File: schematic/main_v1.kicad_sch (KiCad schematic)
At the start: 12 parts

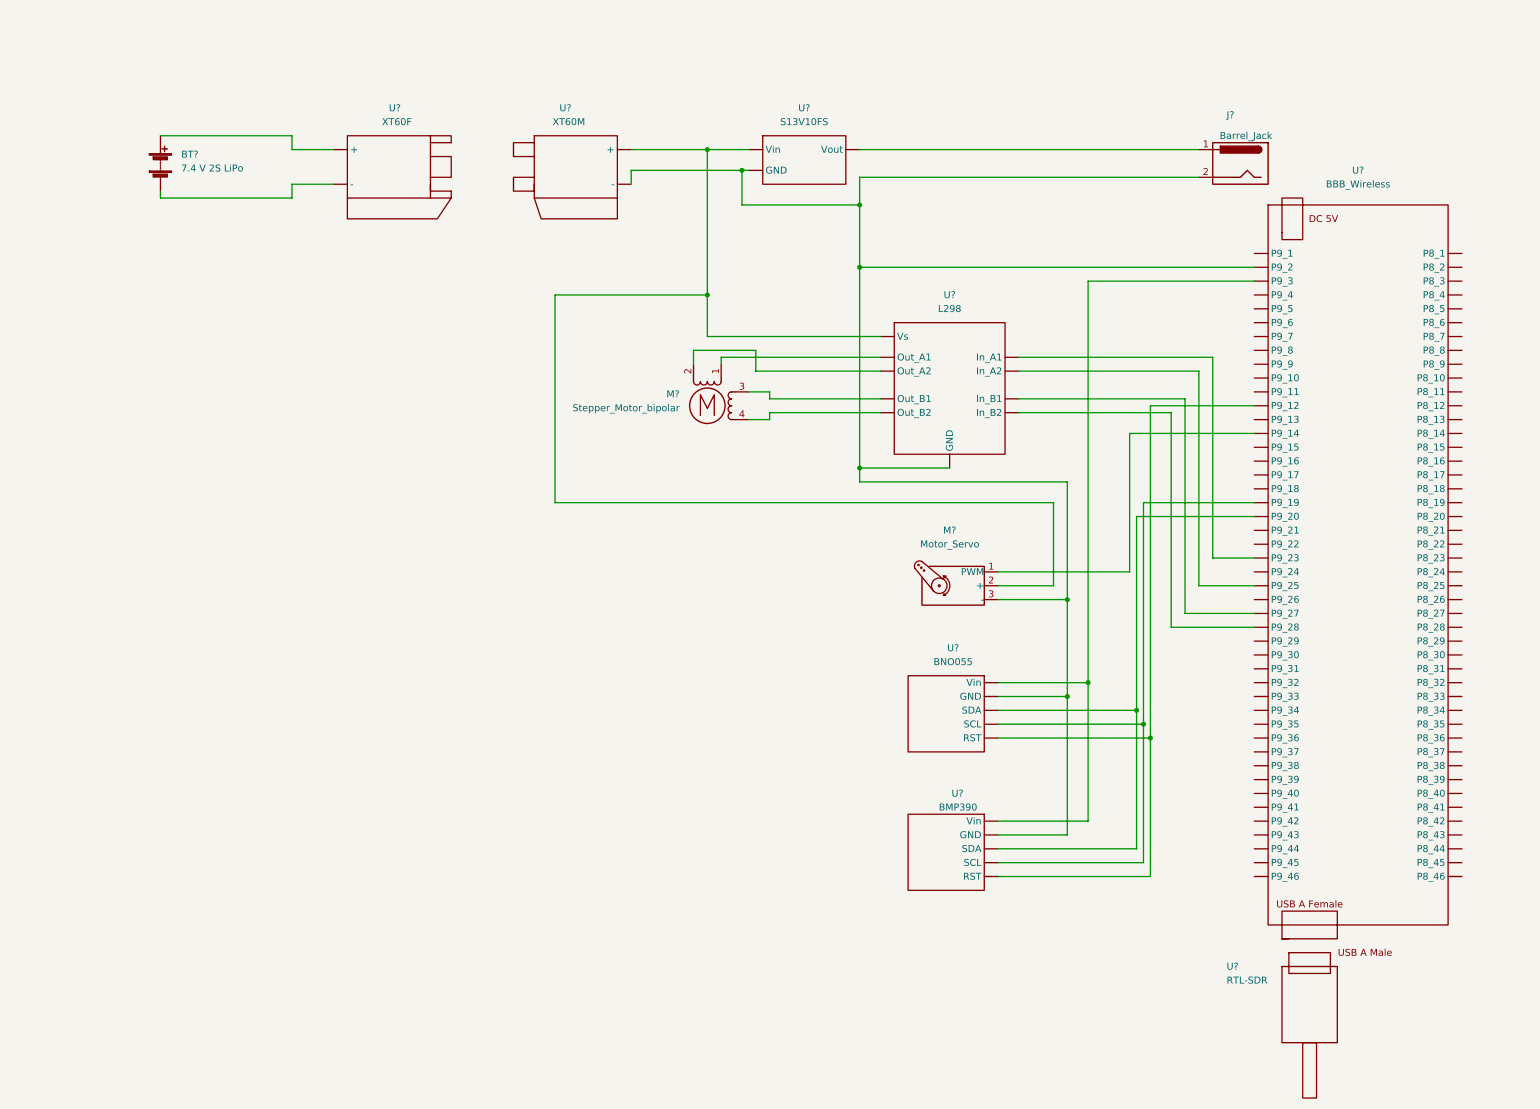
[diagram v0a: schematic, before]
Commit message: Created revision 1.1 of main_v1
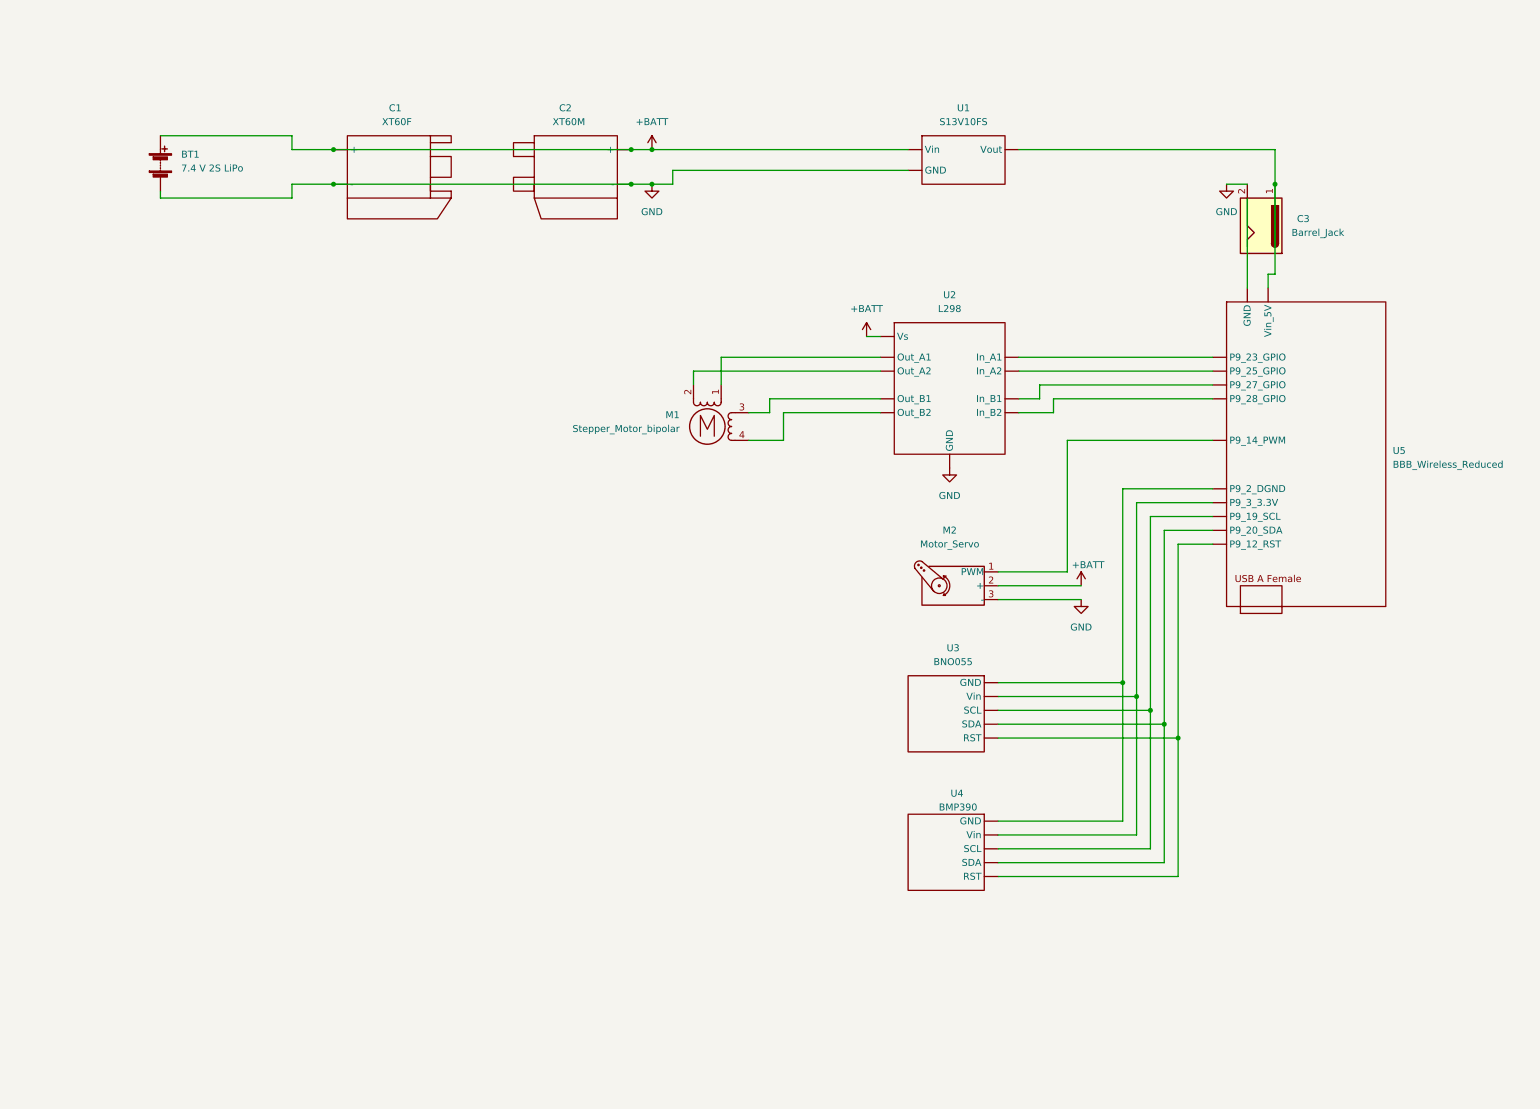
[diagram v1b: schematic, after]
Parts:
- removed U?: RTL-SDR, symbol payload_symbol_library:RTL-SDR
- removed U?: BBB_Wireless, symbol payload_symbol_library:BBB_Wireless
- added U5: BBB_Wireless_Reduced, symbol payload_symbol_library:BBB_Wireless_Reduced
- gave numbers to parts that had none: 10
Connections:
- net GND: now reaches C2. (-), C3.2, M2.3 (-), U1. (Vout), U2. (Vs)
- net GND: now also BT1.2 (-), C1. (-); no longer U3. (Vin), U4. (Vin)
- net at U3. (Vin), U4. (Vin): now also U5. (Vin_5V)
- net at M2.1 (PWM): now also U5. (Vin_5V)
- net at C3.1, U1. (Vout): now also U5. (Vin_5V)
- net +BATT: now reaches BT1.1 (+), C1. (-)
- net +BATT: now also C2. (-), M2.2 (+), U1. (Vout), U2. (Vs)
- new net: U3. (Vin), U4. (Vin), U5. (Vin_5V) (x4)
- new net: U2. (Vs), U5. (Vin_5V) (x4)
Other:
- moved on the sheet: M1, U1

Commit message: main_v1.2 schematic
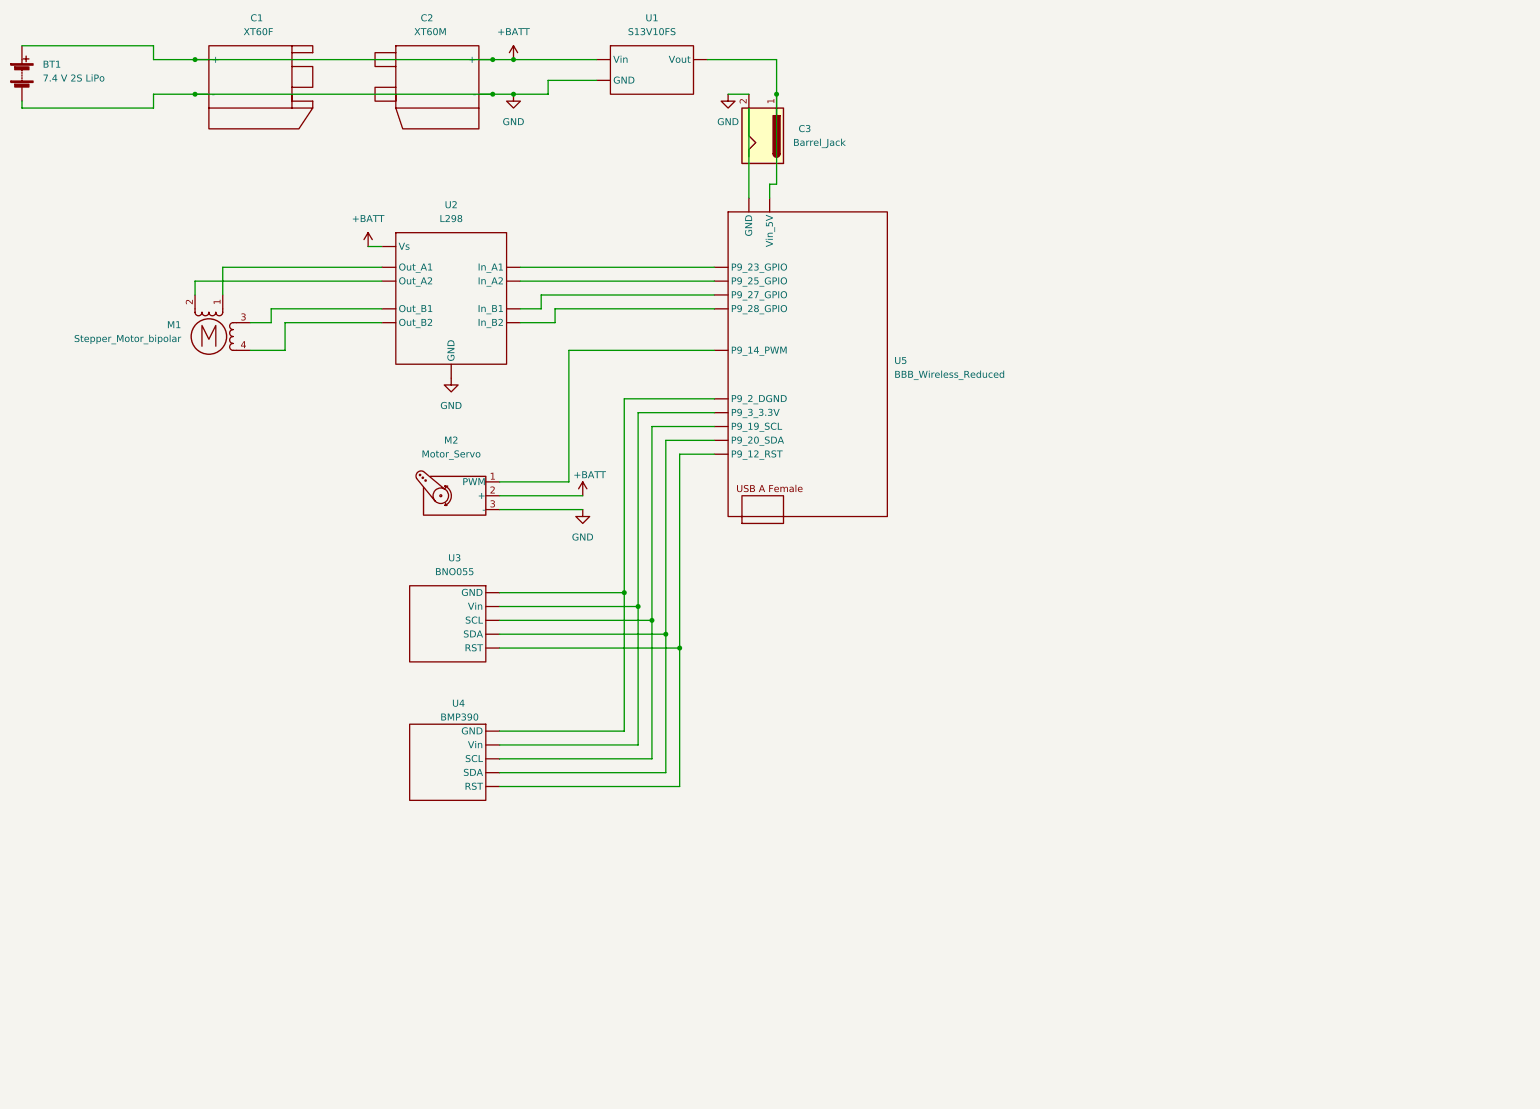
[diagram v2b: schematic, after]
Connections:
- net at U5. (Vin_5V): now also U2. (Vs)
- new net: U3. (Vin), U4. (Vin), U5. (Vin_5V) (x4)
- new net: C3.1, U1. (Vout), U5. (Vin_5V)
- new net: U2. (Vs), U5. (Vin_5V) (x3)
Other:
- moved on the sheet: BT1, C1, C2, C3, M1, M2, U1, U2, U3, U4, U5
